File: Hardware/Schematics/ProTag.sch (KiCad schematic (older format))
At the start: 42 parts, among them IC1 MC3216, IC2 QN9090THN_001Z, J1 Conn_01x01_Female, J2 Conn_01x05_Female, J3 Conn_01x03_Female, J4 Conn_01x02, J5 Conn_01x02, SW1 SW_SPST, U1 TC2185-3.3VxCTTR, Y1 NX2012SA-32.768K-STD-MUB-1, Y2 NX2016SA-32M-EXS00A-CS06465

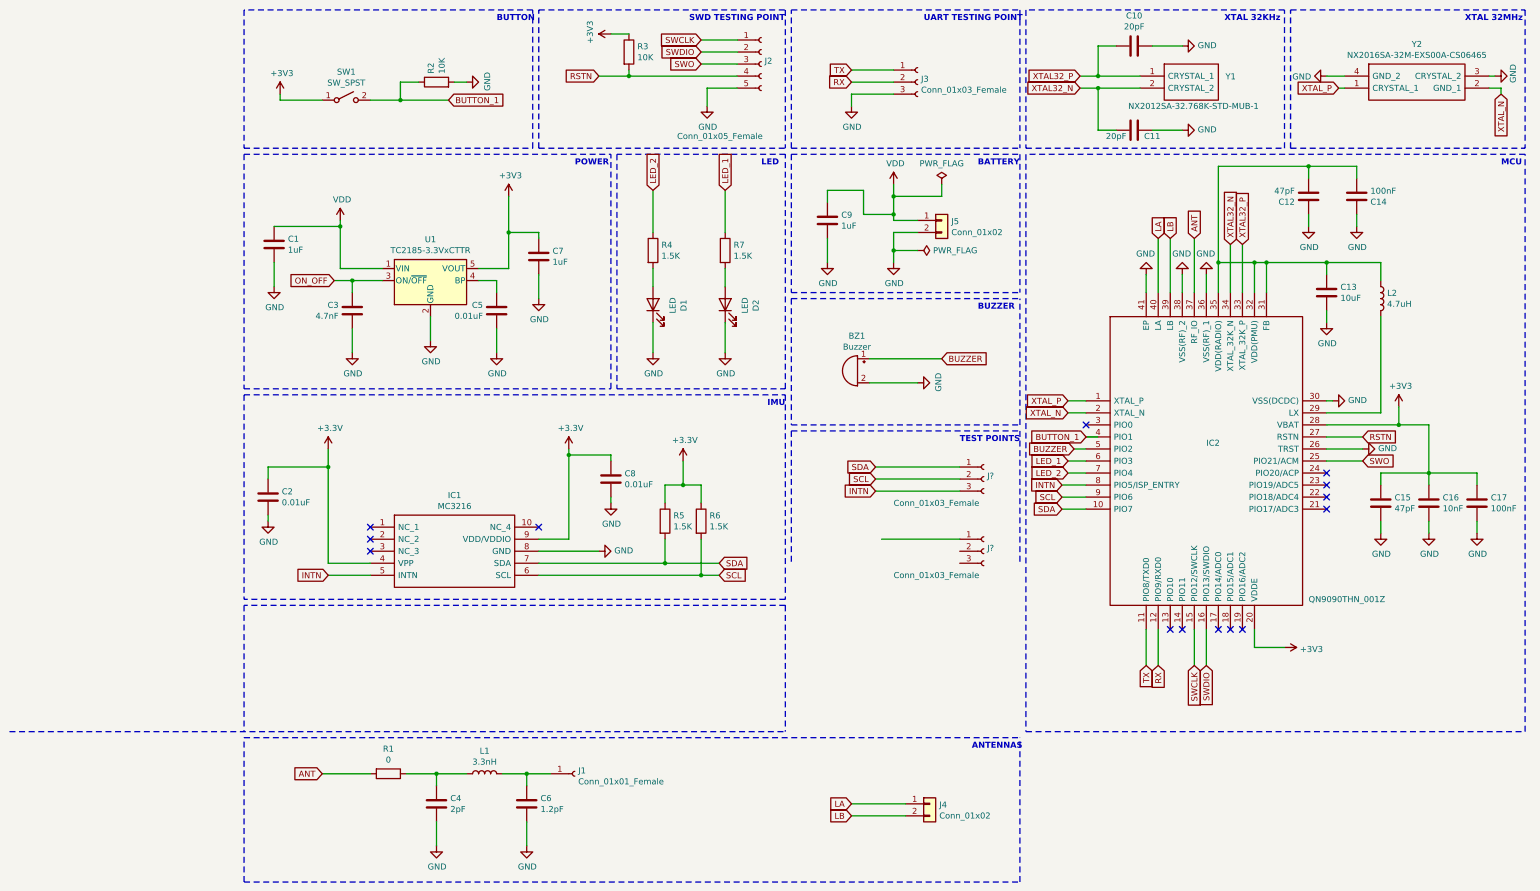
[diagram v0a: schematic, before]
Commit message: Add files via upload
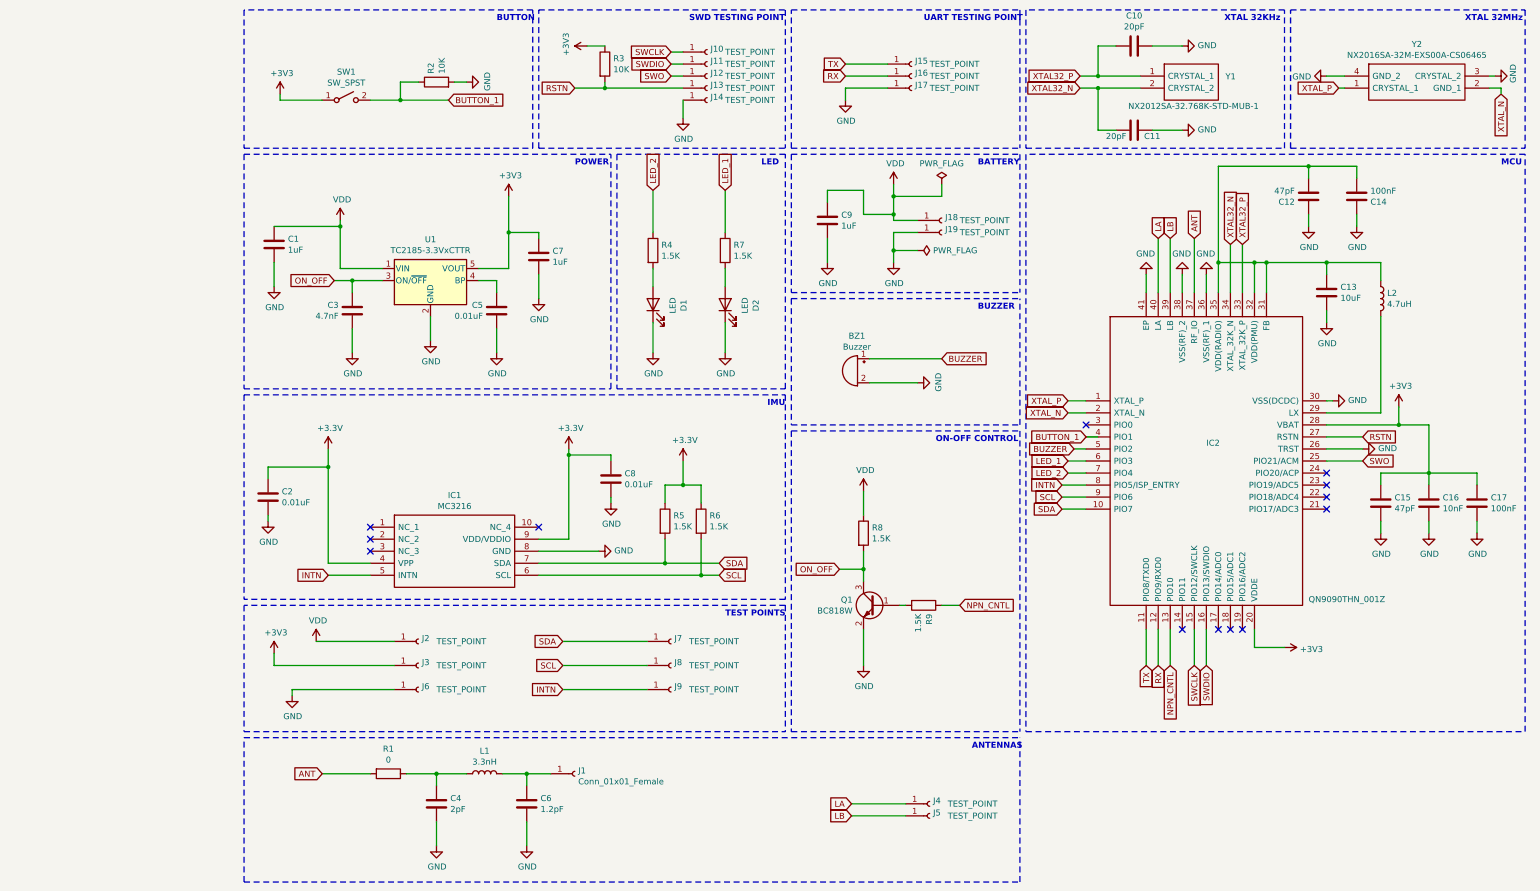
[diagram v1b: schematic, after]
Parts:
- removed J2: Conn_01x05_Female, symbol Connector:Conn_01x05_Female
- removed J3, J? (x2): Conn_01x03_Female, symbol Connector:Conn_01x03_Female
- removed J4, J5: Conn_01x02, symbol Connector_Generic:Conn_01x02
- added J10, J11, J12, J13, J14, J15, J16, J17, J18, J19, J2, J3, J4, J5, J6, J7, J8, J9: TEST_POINT, TestPoint:TestPoint_Pad_D1.0mm, symbol Connector:Conn_01x01_Female
- added Q1: BC818W, Package_TO_SOT_SMD:SOT-323_SC-70, symbol Transistor_BJT:BC818W
- added R8, R9: 1.5K, Resistor_SMD:R_0201_0603Metric, symbol Device:R
- C1, C7, C9: footprint (none) -> Capacitor_SMD:C_0402_1005Metric
- C10, C11, C12, C13, C14, C15, C16, C17, C2, C3, C4, C5, C6, C8: footprint (none) -> Capacitor_SMD:C_0201_0603Metric
- D1, D2: footprint (none) -> Diode_SMD:D_0201_0603Metric
- J1: footprint (none) -> TestPoint:TestPoint_Pad_D1.0mm
- L1, L2: footprint (none) -> Inductor_SMD:L_0201_0603Metric
- R1, R2, R3, R4, R5, R6, R7: footprint (none) -> Resistor_SMD:R_0201_0603Metric
- SW1: footprint (none) -> Button_Switch_SMD:SW_SPST_TL3342
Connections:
- net +3V3: now also J3.1 (Pin_1)
- net GND: now also J14.1 (Pin_1), J17.1 (Pin_1), J19.1 (Pin_1), J6.1 (Pin_1), Q1.2 (E)
- net INTN: now also J9.1 (Pin_1)
- net LA: now also J4.1 (Pin_1)
- net LB: now also J5.1 (Pin_1)
- net ON_OFF: now also Q1.3 (C), R8.2
- net RSTN: now also J13.1 (Pin_1)
- net RX: now also J16.1 (Pin_1)
- net SCL: now also J8.1 (Pin_1)
- net SDA: now also J7.1 (Pin_1)
- net SWCLK: now also J10.1 (Pin_1)
- net SWDIO: now also J11.1 (Pin_1)
- net SWO: now also J12.1 (Pin_1)
- net TX: now also J15.1 (Pin_1)
- net VDD: now also J18.1 (Pin_1), J2.1 (Pin_1), R8.1
- net NPN_CNTL: now reaches IC2.13 (PIO10)
- net NPN_CNTL: now also R9.1
- new net: Q1.1 (B), R9.2
- no-connect marks 14 -> 13
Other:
- note added: "ON-OFF CONTROL"
- moved on the sheet: R3
